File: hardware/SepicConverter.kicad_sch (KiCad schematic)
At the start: 11 parts, among them J3 Conn_01x04 5.08mm, J4 Conn_01x04 5.08mm, Q1 IRF640N, U4 TC4422

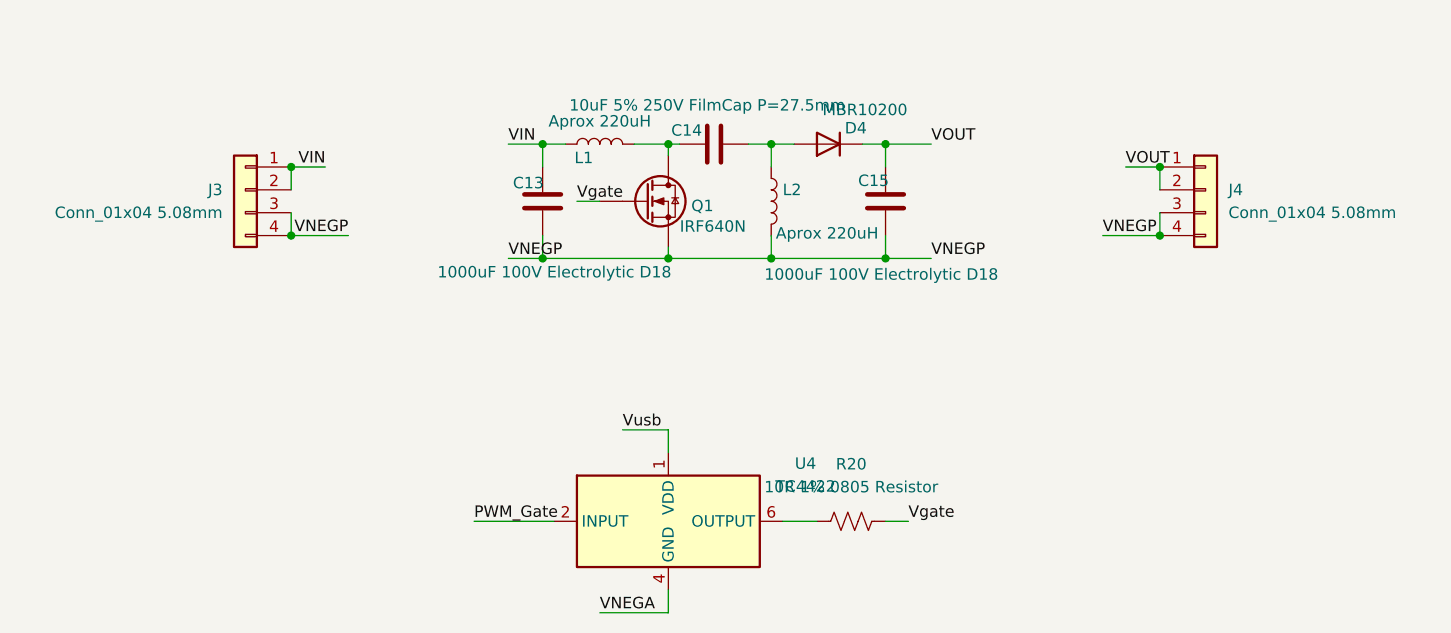
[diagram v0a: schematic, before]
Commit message: HW: sch near final version
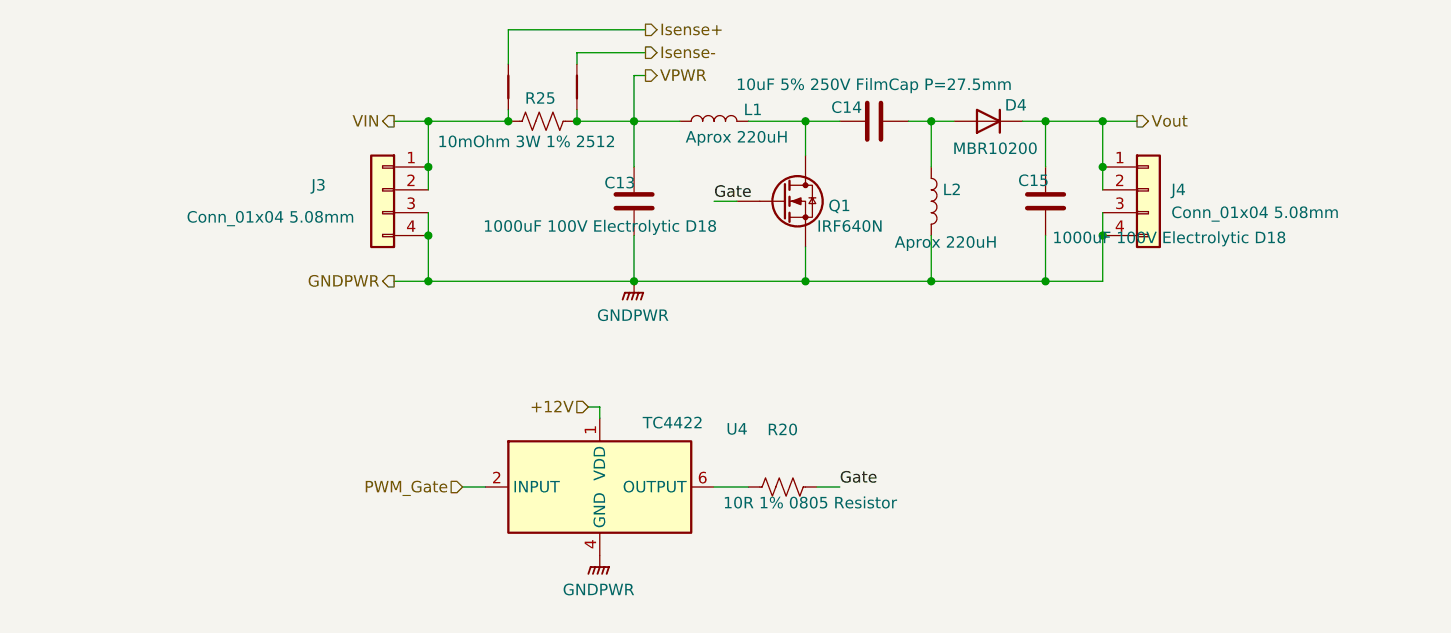
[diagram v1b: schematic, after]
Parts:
- added NT1, NT2: NetTie_2, NetTie:NetTie-2_SMD_Pad2.0mm, symbol Device:NetTie_2
- added R25: 10mOhm 3W 1% 2512, Resistor_SMD:R_2512_6332Metric_Pad1.40x3.35mm_HandSolder, symbol Device:R_US
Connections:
- net VNEGP is gone; now on net GNDPWR: C13.2, C15.1, J3.3 (Pin_3), J3.4 (Pin_4), J4.3 (Pin_3), J4.4 (Pin_4), L2.2, Q1.S
- net VIN: now also NT1.1, R25.1; no longer C13.1, L1.1
- net VNEGA renamed GNDPWR
- net VOUT renamed Vout
- net Vgate renamed Gate
- net Vusb renamed +12V
- new net Isense+: NT1.2
- new net Isense-: NT2.2
- new net VPWR: C13.1, L1.1, NT2.1, R25.2
